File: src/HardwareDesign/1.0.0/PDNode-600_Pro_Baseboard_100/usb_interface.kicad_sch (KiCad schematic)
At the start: 13 parts, among them IC3 FSUSB42MUX, J3 USB-TYPE-C-018

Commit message: M54 rework
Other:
- company: DvidMakesThings -> ${COMPANY}
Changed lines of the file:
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@@
 	(title_block
 		(title "USB Interface")
-		(date "2026-02-05")
-		(rev "1.0.0")
-		(company "DvidMakesThings")
+		(date "2025-01-12")
+		(rev "${REVISION}")
+		(company "${COMPANY}")
 	)
 	(text "USB DATA-PATH SELECTOR"

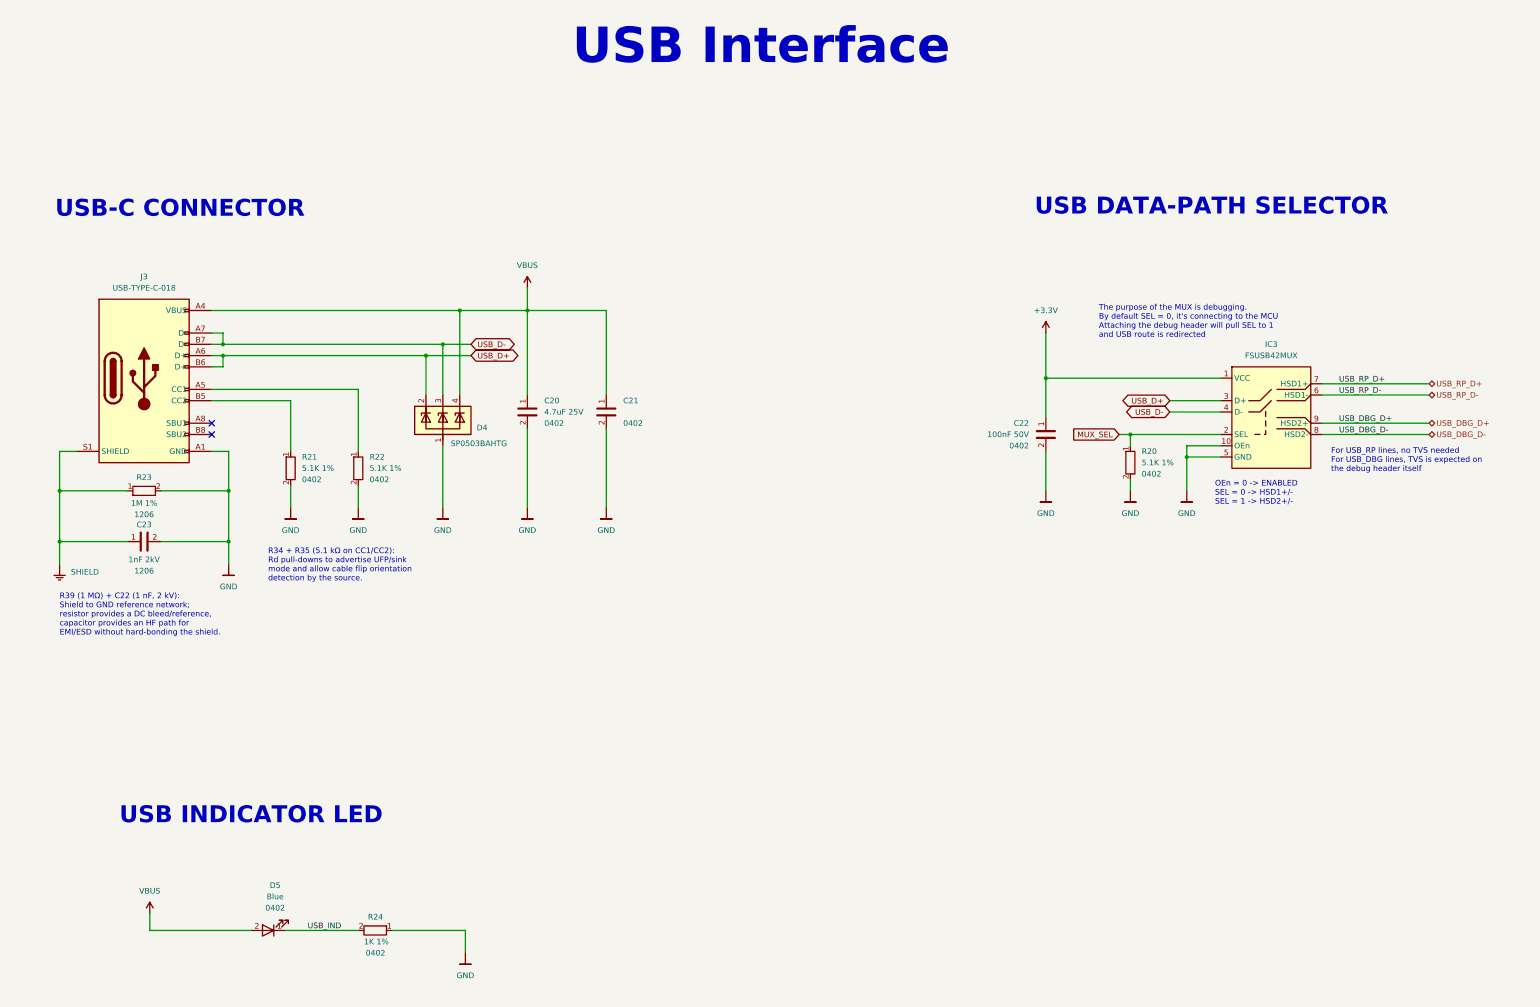
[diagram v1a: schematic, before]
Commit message: baseboard development
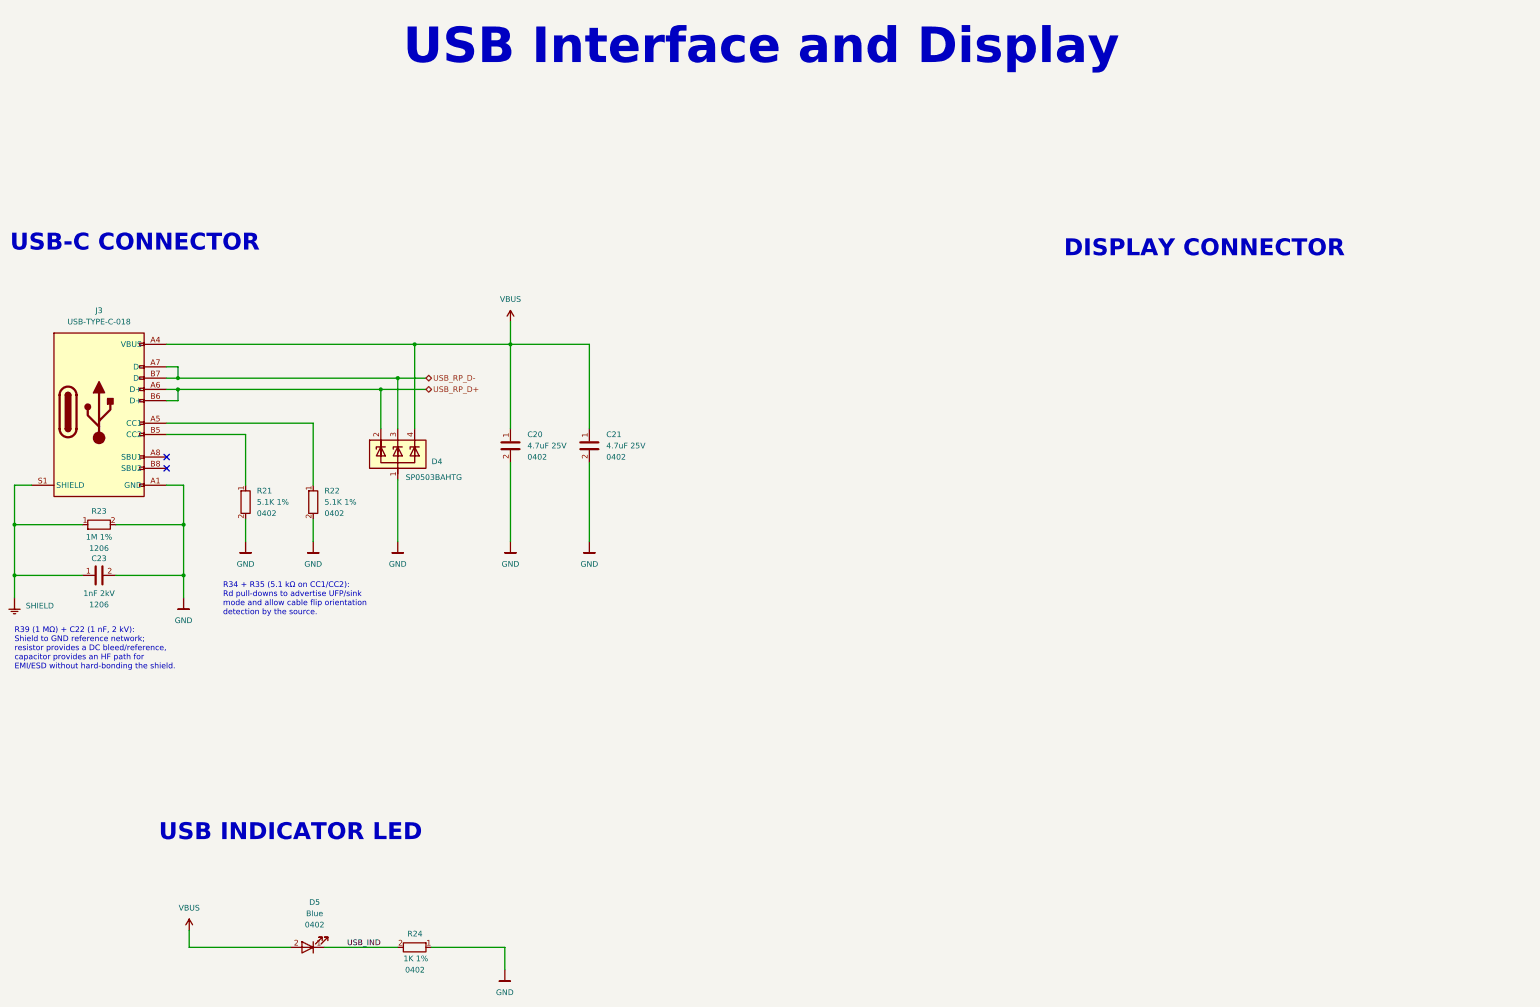
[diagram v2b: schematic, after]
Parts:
- removed C22: 100nF 50V, Capacitor_SMD:C_0402_1005Metric, symbol DS_Capacitor_0402:100nF 50V 0402
- removed IC3: FSUSB42MUX, DS_Peripherals:MSOP-10_3x3mm_P0.5mm, symbol DS_Peripherals:FSUSB42MUX
- removed R20: 5.1K 1%, Resistor_SMD:R_0402_1005Metric, symbol DS_Resistor_0402:5.1K 1% 0402
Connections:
- net USB_D+ is gone; now on net USB_RP_D+: D4.2, J3.A6 (D+), J3.B6 (D+)
- net USB_D- is gone; now on net USB_RP_D-: D4.3, J3.A7 (D-), J3.B7 (D-)
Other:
- note added: "DISPLAY CONNECTOR"
- note removed: "For USB_RP lines, no TVS needed For USB_DBG lines, TVS is expected on the debug header itself"
- note removed: "OEn = 0 -> ENABLED SEL = 0 -> HSD1+/- SEL = 1 -> HSD2+/-"
- note removed: "The purpose of the MUX is debugging. By default SEL = 0, it's connecting to the MCU Attaching the debug header will pull SEL to 1 and USB route is redirected"
- note removed: "USB DATA-PATH SELECTOR"
- moved on the sheet: C20, C21, C23, D4, D5, J3, R21, R22, R23, R24
